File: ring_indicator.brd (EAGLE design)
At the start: 56.8 x 36.8 mm, 21 parts, among them Q2 BUZ11

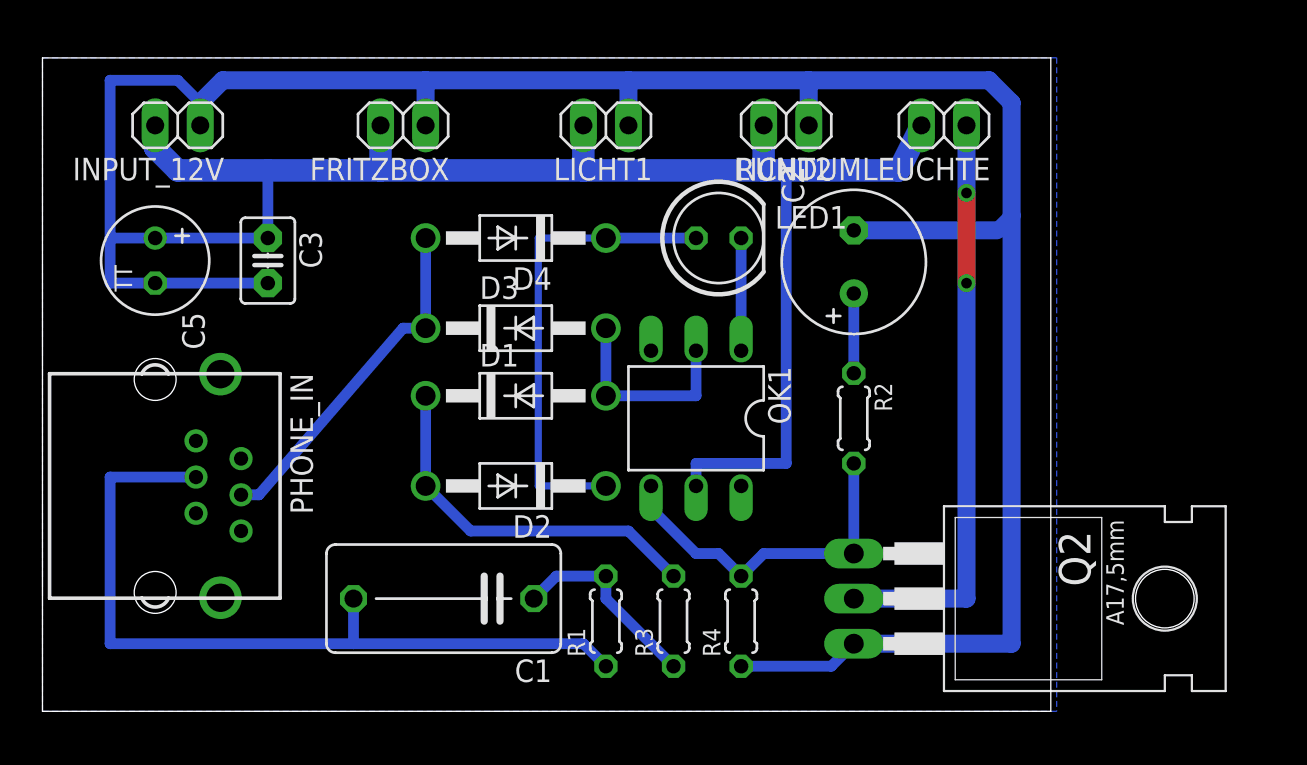
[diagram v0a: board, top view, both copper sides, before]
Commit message: v0.2-produced
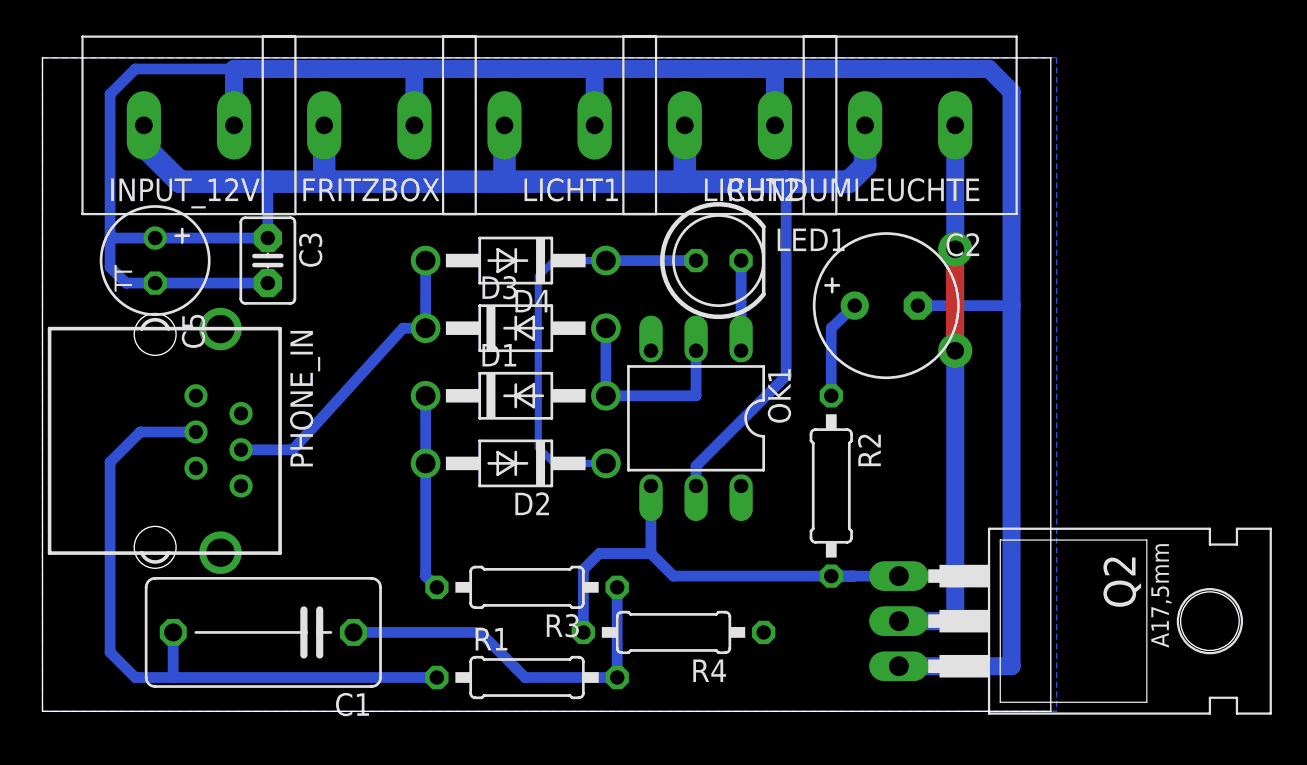
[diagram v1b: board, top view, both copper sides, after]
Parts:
- FRITZBOX, INPUT_12V, LICHT1, LICHT2, RUNDUMLEUCHTE: value (none) -> CON_23.81; device pinhead:1X02 -> pcaroli:CON_2_3.81
- R1, R2, R3, R4: device rcl:0204/5 -> rcl:0207/10
- moved C1 10.3 mm to (12.4, 4.45)
- moved R3 8.47 mm to (27.3, 6.99), turned to 180 degrees
- moved R1 5.46 mm to (27.3, 1.91), turned to 0 degrees
- moved R2 4.02 mm to (44.5, 12.7)
- moved R4 3.86 mm to (35.6, 4.45), turned to 180 degrees
- moved LICHT1 3.18 mm to (28.6, 33.0)
- moved LICHT2 3.17 mm to (38.7, 33.0)
- moved C2 3.07 mm to (47.5, 22.9), turned to 0 degrees
- moved Q2 2.84 mm to (54.6, 5.08)
- moved PHONE_IN 2.54 mm to (6.35, 15.2)
- moved FRITZBOX 1.91 mm to (18.4, 33.0)
- moved RUNDUMLEUCHTE 1.90 mm to (48.9, 33.0)
- moved D4 1.27 mm to (26.7, 25.4)
- moved LED1 1.27 mm to (38.1, 25.4)
- moved D2 1.27 mm to (26.7, 14.0)
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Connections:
- net GND: now also FRITZBOX.P$1, INPUT_12V.P$1, LICHT1.P$1, LICHT2.P$1; no longer FRITZBOX.1, INPUT_12V.1, LICHT1.1, LICHT2.1
- net N$6: now also RUNDUMLEUCHTE.P$1; no longer RUNDUMLEUCHTE.1
- net VCC: now also FRITZBOX.P$2, INPUT_12V.P$2, LICHT1.P$2, LICHT2.P$2, RUNDUMLEUCHTE.P$2; no longer FRITZBOX.2, INPUT_12V.2, LICHT1.2, LICHT2.2, RUNDUMLEUCHTE.2
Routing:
- net N$3: track 21.2 -> 11.1 mm
- net N$1: track 11.2 -> 21.0 mm
- net GND: track 139.6 -> 130.2 mm
- net A: track 45.2 -> 37.8 mm
- net N$9: track 19.9 -> 27.3 mm
- net VCC: track 87.2 -> 83.6 mm
- net N$4: track 26.7 -> 23.1 mm
- net B: track 19.8 -> 17.2 mm
- net N$6: track 33.0 -> 31.1 mm
- net N$2: track 6.35 -> 5.08 mm
- net N$10: track 4.50 -> 5.64 mm
